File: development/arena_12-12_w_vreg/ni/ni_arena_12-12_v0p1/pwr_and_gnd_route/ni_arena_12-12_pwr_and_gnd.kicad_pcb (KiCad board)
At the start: 6 copper layers, 228.6 x 228.6 mm, 126 parts, among them J1 Barrel_Jack, J2 NI_TE_68pos, P1 CONN15, P10 CONN15, P11 CONN15, P12 CONN15, P2 CONN15, P3 CONN15, P4 CONN15, P5 CONN15, P6 CONN15, P7 CONN15, P8 CONN15, P9 CONN15, Q2 MOSFET_NCHAN, SW1 SW_SPDT, U1 TXB0108PW, U10 TPS564201DDC, U11 TPS564201DDC, U12 TPS564201DDC, U13 TPS564201DDC, U14 TPS564201DDC, U15 TPS564201DDC, U16 TPS564201DDC, U17 TPS564201DDC, U18 AP2112K-3.3, U2 TXB0108PW, U3 TXB0108PW, U4 TXB0108PW, U5 TXB0108PW, U6 TPS564201DDC, U7 TPS564201DDC, U8 TPS564201DDC, U9 TPS564201DDC

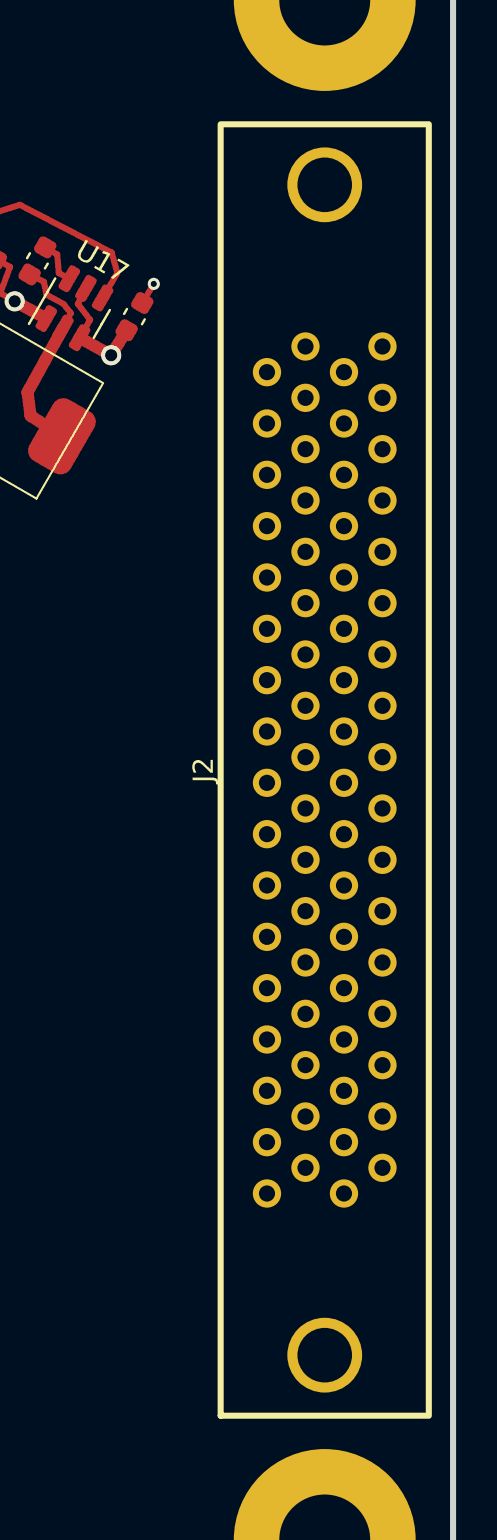
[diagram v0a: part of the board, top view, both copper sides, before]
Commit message: Intermediate save during re-route of NI 12-12 arena with vreg.
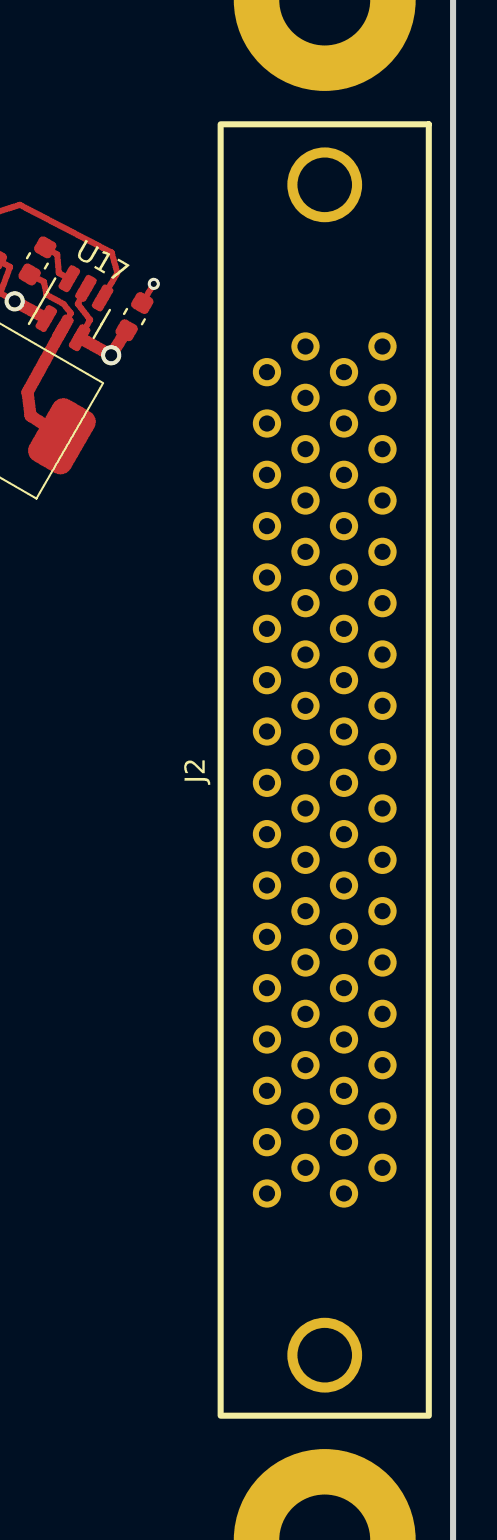
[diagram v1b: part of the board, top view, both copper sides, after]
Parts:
- turned J2 to -90 degrees
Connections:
- J2 pad 35: /Level Shifters/PAN3V.EXT_INT -> /Level Shifters/PAN3V.CS_00
- J2 pad 36: /Level Shifters/PAN3V.MISO_11 -> /Level Shifters/PAN3V.CS_01
- J2 pad 37: /Level Shifters/PAN3V.MISO_10 -> /Level Shifters/PAN3V.CS_02
- J2 pad 38: /Level Shifters/PAN3V.MISO_09 -> /Level Shifters/PAN3V.CS_03
- J2 pad 39: /Level Shifters/PAN3V.MISO_08 -> /Level Shifters/PAN3V.CS_04
- J2 pad 40: /Level Shifters/PAN3V.MISO_07 -> /Level Shifters/PAN3V.CS_05
- J2 pad 41: /Level Shifters/PAN3V.MISO_06 -> /Level Shifters/PAN3V.CS_06
- J2 pad 42: /Level Shifters/PAN3V.MOSI_06 -> /Level Shifters/PAN3V.CS_07
- J2 pad 43: /Level Shifters/PAN3V.MISO_05 -> /Level Shifters/PAN3V.SCK_00
- J2 pad 44: /Level Shifters/PAN3V.MOSI_05 -> /Level Shifters/PAN3V.SCK_01
- J2 pad 45: /Level Shifters/PAN3V.MISO_04 -> /Level Shifters/PAN3V.SCK_02
- J2 pad 46: /Level Shifters/PAN3V.MOSI_04 -> /Level Shifters/PAN3V.SCK_03
- J2 pad 47: /Level Shifters/PAN3V.MISO_03 -> /Level Shifters/PAN3V.SCK_04
- J2 pad 48: /Level Shifters/PAN3V.MOSI_03 -> /Level Shifters/PAN3V.SCK_05
- J2 pad 49: /Level Shifters/PAN3V.MISO_02 -> /Level Shifters/PAN3V.MOSI_00
- J2 pad 50: /Level Shifters/PAN3V.MOSI_02 -> /Level Shifters/PAN3V.MISO_00
- J2 pad 51: /Level Shifters/PAN3V.MISO_01 -> /Level Shifters/PAN3V.MOSI_01
- J2 pad 52: /Level Shifters/PAN3V.MOSI_01 -> /Level Shifters/PAN3V.MISO_01
- J2 pad 53: /Level Shifters/PAN3V.MISO_00 -> /Level Shifters/PAN3V.MOSI_02
- J2 pad 54: /Level Shifters/PAN3V.MOSI_00 -> /Level Shifters/PAN3V.MISO_02
- J2 pad 55: /Level Shifters/PAN3V.SCK_05 -> /Level Shifters/PAN3V.MOSI_03
- J2 pad 56: /Level Shifters/PAN3V.SCK_04 -> /Level Shifters/PAN3V.MISO_03
- J2 pad 57: /Level Shifters/PAN3V.SCK_03 -> /Level Shifters/PAN3V.MOSI_04
- J2 pad 58: /Level Shifters/PAN3V.SCK_02 -> /Level Shifters/PAN3V.MISO_04
- J2 pad 59: /Level Shifters/PAN3V.SCK_01 -> /Level Shifters/PAN3V.MOSI_05
- J2 pad 60: /Level Shifters/PAN3V.SCK_00 -> /Level Shifters/PAN3V.MISO_05
- J2 pad 61: /Level Shifters/PAN3V.CS_07 -> /Level Shifters/PAN3V.MOSI_06
- J2 pad 62: /Level Shifters/PAN3V.CS_06 -> /Level Shifters/PAN3V.MISO_06
- J2 pad 63: /Level Shifters/PAN3V.CS_05 -> /Level Shifters/PAN3V.MISO_07
- J2 pad 64: /Level Shifters/PAN3V.CS_04 -> /Level Shifters/PAN3V.MISO_08
- J2 pad 65: /Level Shifters/PAN3V.CS_03 -> /Level Shifters/PAN3V.MISO_09
- J2 pad 66: /Level Shifters/PAN3V.CS_02 -> /Level Shifters/PAN3V.MISO_10
- J2 pad 67: /Level Shifters/PAN3V.CS_01 -> /Level Shifters/PAN3V.MISO_11
- J2 pad 68: /Level Shifters/PAN3V.CS_00 -> /Level Shifters/PAN3V.EXT_INT
